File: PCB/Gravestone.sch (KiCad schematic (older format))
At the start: 30 parts, among them J1 USB_C_Receptacle_USB2.0, SW1 SW_PUSH, U1 ATmega32U2-AU, Y1 16MHz

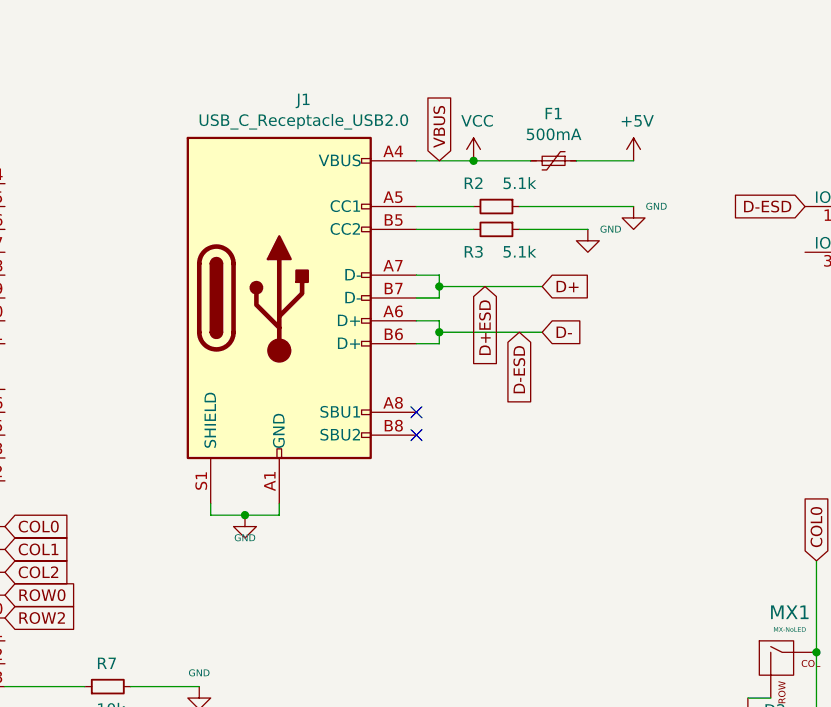
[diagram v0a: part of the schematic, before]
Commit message: 9/07 usb2
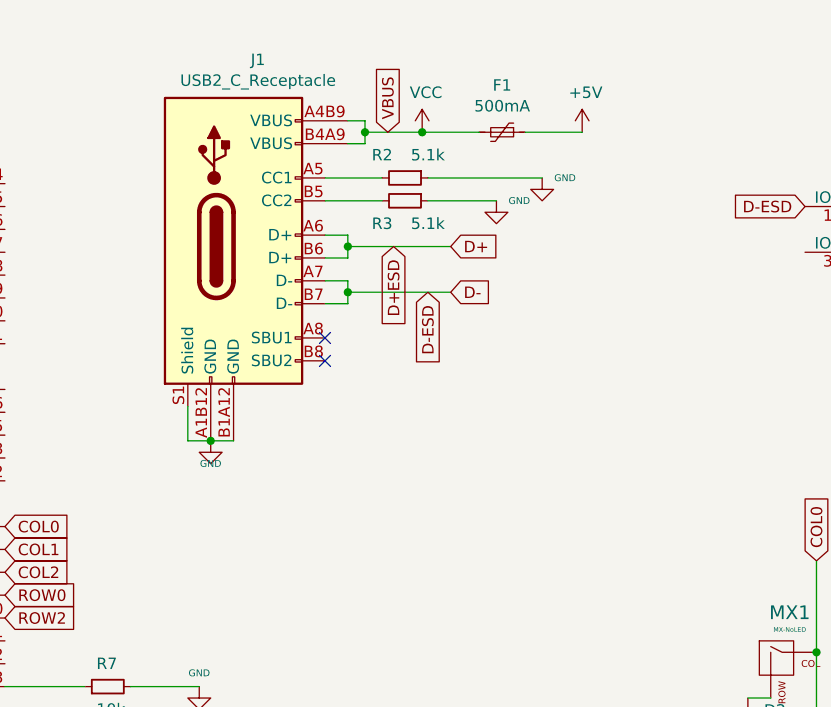
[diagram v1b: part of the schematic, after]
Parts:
- removed J1: USB_C_Receptacle_USB2.0, usb-type-c:Mid_Mount-USB_C_HandSoldering, symbol Connector:USB_C_Receptacle_USB2.0
- added J1: USB2_C_Receptacle, usb-type-c:Mid_Mount-USB_C_HandSoldering, symbol usb-type-c:USB2_C_Receptacle
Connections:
- net D+: now also J1.A6 (D+), J1.B6 (D+)
- net D-: now also J1.A7 (D-), J1.B7 (D-)
- net GND: now also J1.A1B12 (GND), J1.B1A12 (GND), J1.S1 (Shield)
- net VCC: now also J1.A4B9 (VBUS), J1.B4A9 (VBUS)
- net at R2.2: now also J1.A5 (CC1)
- net at R3.2: now also J1.B5 (CC2)
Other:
- moved on the sheet: F1, R2, R3
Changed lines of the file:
@@
 L Device:R_Small R2
 U 1 1 5F466C25
-P 6050 1650
-F 0 "R2" V 5950 1550 50  0000 C CNN
-F 1 "5.1k" V 5950 1750 50  0000 C CNN
-F 2 "Keebio-Parts:R_0603" H 6050 1650 50  0001 C CNN
-F 3 "~" H 6050 1650 50  0001 C CNN
-	1    6050 1650
+P 5650 1525
+F 0 "R2" V 5550 1425 50  0000 C CNN
+F 1 "5.1k" V 5550 1625 50  0000 C CNN
+F 2 "Keebio-Parts:R_0603" H 5650 1525 50  0001 C CNN
+F 3 "~" H 5650 1525 50  0001 C CNN
+	1    5650 1525
 	0    1    1    0
 $EndComp
@@
 	2400 1250 2400 1150
 $Comp
-L Connector:USB_C_Receptacle_USB2.0 J1
-U 1 1 5F45EACB
-P 5100 2050
-F 0 "J1" H 5207 2917 50  0000 C CNN
-F 1 "USB_C_Receptacle_USB2.0" H 5207 2826 50  0000 C CNN
-F 2 "usb-type-c:Mid_Mount-USB_C_HandSoldering" H 5250 2050 50  0001 C CNN
-F 3 "https://www.usb.org/sites/default/files/documents/usb_type-c.zip" H 5250 2050 50  0001 C CNN
-	1    5100 2050
-	1    0    0    -1
-$EndComp
-$Comp
 L power:GND #PWR0111
 U 1 1 5F461E03
-P 4950 3000
-F 0 "#PWR0111" H 4950 3050 20  0001 C CNN
-F 1 "GND" H 4950 2900 30  0000 C CNN
-F 2 "" H 4950 3000 60  0000 C CNN
-F 3 "" H 4950 3000 60  0000 C CNN
-	1    4950 3000
+P 4800 2675
+F 0 "#PWR0111" H 4800 2725 20  0001 C CNN
+F 1 "GND" H 4800 2575 30  0000 C CNN
+F 2 "" H 4800 2675 60  0000 C CNN
+F 3 "" H 4800 2675 60  0000 C CNN
+	1    4800 2675
 	1    0    0    -1
 $EndComp
@@
 L power:VCC #PWR0112
 U 1 1 5F46330E
-P 5950 1450
-F 0 "#PWR0112" H 5950 1300 50  0001 C CNN
-F 1 "VCC" H 5967 1623 50  0000 C CNN
-F 2 "" H 5950 1450 50  0001 C CNN
-F 3 "" H 5950 1450 50  0001 C CNN
-	1    5950 1450
+P 5725 1325
+F 0 "#PWR0112" H 5725 1175 50  0001 C CNN
+F 1 "VCC" H 5742 1498 50  0000 C CNN
+F 2 "" H 5725 1325 50  0001 C CNN
+F 3 "" H 5725 1325 50  0001 C CNN
+	1    5725 1325
 	1    0    0    -1
 $EndComp
@@
 L Device:Polyfuse_Small F1
 U 1 1 5F464504
-P 6300 1450
-F 0 "F1" V 6095 1450 50  0000 C CNN
-F 1 "500mA" V 6186 1450 50  0000 C CNN
-F 2 "Fuse:Fuse_0805_2012Metric" H 6350 1250 50  0001 L CNN
-F 3 "~" H 6300 1450 50  0001 C CNN
-	1    6300 1450
+P 6075 1325
+F 0 "F1" V 5870 1325 50  0000 C CNN
+F 1 "500mA" V 5961 1325 50  0000 C CNN
+F 2 "Fuse:Fuse_0805_2012Metric" H 6125 1125 50  0001 L CNN
+F 3 "~" H 6075 1325 50  0001 C CNN
+	1    6075 1325
 	0    1    1    0
 $EndComp
@@
 L power:+5V #PWR0113
 U 1 1 5F465DF5
-P 6650 1450
-F 0 "#PWR0113" H 6650 1300 50  0001 C CNN
-F 1 "+5V" H 6665 1623 50  0000 C CNN
-F 2 "" H 6650 1450 50  0001 C CNN
-F 3 "" H 6650 1450 50  0001 C CNN
-	1    6650 1450
-	1    0    0    -1
-$EndComp
-Wire Wire Line
-	5700 1450 5950 1450
-Wire Wire Line
-	6400 1450 6650 1450
-Connection ~ 5950 1450
-Wire Wire Line
-	5950 1450 6200 1450
+P 6425 1325
+F 0 "#PWR0113" H 6425 1175 50  0001 C CNN
+F 1 "+5V" H 6440 1498 50  0000 C CNN
+F 2 "" H 6425 1325 50  0001 C CNN
+F 3 "" H 6425 1325 50  0001 C CNN
+	1    6425 1325
+	1    0    0    -1
+$EndComp
+Wire Wire Line
+	5475 1325 5725 1325
+Wire Wire Line
+	6175 1325 6425 1325
+Connection ~ 5725 1325
+Wire Wire Line
+	5725 1325 5975 1325
 $Comp
 L Device:R_Small R3
 U 1 1 5F468C9D
-P 6050 1750
-F 0 "R3" V 6150 1650 50  0000 C CNN
-F 1 "5.1k" V 6150 1850 50  0000 C CNN
-F 2 "Keebio-Parts:R_0603" H 6050 1750 50  0001 C CNN
-F 3 "~" H 6050 1750 50  0001 C CNN
-	1    6050 1750
-	0    1    1    0
-$EndComp
-Wire Wire Line
-	5700 1650 5950 1650
-Wire Wire Line
-	5700 1750 5950 1750
+P 5650 1625
+F 0 "R3" V 5750 1525 50  0000 C CNN
+F 1 "5.1k" V 5750 1725 50  0000 C CNN
+F 2 "Keebio-Parts:R_0603" H 5650 1625 50  0001 C CNN
+F 3 "~" H 5650 1625 50  0001 C CNN
+	1    5650 1625
+	0    1    1    0
+$EndComp
+Wire Wire Line
+	5300 1525 5550 1525
+Wire Wire Line
+	5300 1625 5550 1625
 $Comp
 L Power_Protection:SRV05-4 D1
@@
 $EndComp
 Wire Wire Line
-	5700 1950 5800 1950
-Wire Wire Line
-	5800 2050 5700 2050
-Wire Wire Line
-	5700 2150 5800 2150
-Wire Wire Line
-	5800 2250 5700 2250
-Text GLabel 6250 2000 2    50   Input ~ 0
+	5300 1775 5400 1775
+Wire Wire Line
+	5400 1875 5300 1875
+Wire Wire Line
+	5300 1975 5400 1975
+Wire Wire Line
+	5400 2075 5300 2075
+Text GLabel 5850 1825 2    50   Input ~ 0
 D+
-Text GLabel 6250 2200 2    50   Input ~ 0
+Text GLabel 5850 2025 2    50   Input ~ 0
 D-
-NoConn ~ 5700 2550
-NoConn ~ 5700 2650
-Wire Wire Line
-	5100 2950 5100 3000
+NoConn ~ 5300 2225
+NoConn ~ 5300 2325
 $Comp
 L Gravestone-rescue:MX-NoLED-MX_Alps_Hybrid MX1
@@
 Wire Wire Line
 	3100 4150 3200 4150
-Wire Wire Line
-	4800 2950 4800 3000
 $Comp
 L power:GND #PWR0114
 U 1 1 5F56CBA5
-P 6650 1650
-F 0 "#PWR0114" H 6650 1700 20  0001 C CNN
-F 1 "GND" H 6750 1650 30  0000 C CNN
-F 2 "" H 6650 1650 60  0000 C CNN
-F 3 "" H 6650 1650 60  0000 C CNN
-	1    6650 1650
-	1    0    0    -1
-$EndComp
-Wire Wire Line
-	4800 3000 4950 3000
-Connection ~ 4950 3000
-Wire Wire Line
-	4950 3000 5100 3000
-Text GLabel 5800 1450 1    50   Input ~ 0
+P 6250 1525
+F 0 "#PWR0114" H 6250 1575 20  0001 C CNN
+F 1 "GND" H 6350 1525 30  0000 C CNN
+F 2 "" H 6250 1525 60  0000 C CNN
+F 3 "" H 6250 1525 60  0000 C CNN
+	1    6250 1525
+	1    0    0    -1
+$EndComp
+Text GLabel 5575 1325 1    50   Input ~ 0
 VBUS
 Wire Wire Line
-	5800 1950 5800 2000
-Wire Wire Line
-	5800 2150 5800 2200
+	5400 1775 5400 1825
+Wire Wire Line
+	5400 1975 5400 2025
 $Comp
 L power:GND #PWR0115
 U 1 1 5F48A564
-P 6450 1750
-F 0 "#PWR0115" H 6450 1800 20  0001 C CNN
-F 1 "GND" H 6550 1750 30  0000 C CNN
-F 2 "" H 6450 1750 60  0000 C CNN
-F 3 "" H 6450 1750 60  0000 C CNN
-	1    6450 1750
-	1    0    0    -1
-$EndComp
-Wire Wire Line
-	6150 1650 6650 1650
-Wire Wire Line
-	6150 1750 6450 1750
-Connection ~ 5800 2000
-Wire Wire Line
-	5800 2000 5800 2050
-Connection ~ 5800 2200
-Wire Wire Line
-	5800 2200 5800 2250
-Text GLabel 6150 2200 3    50   Input ~ 0
+P 6050 1625
+F 0 "#PWR0115" H 6050 1675 20  0001 C CNN
+F 1 "GND" H 6150 1625 30  0000 C CNN
+F 2 "" H 6050 1625 60  0000 C CNN
+F 3 "" H 6050 1625 60  0000 C CNN
+	1    6050 1625
+	1    0    0    -1
+$EndComp
+Wire Wire Line
+	5750 1525 6250 1525
+Wire Wire Line
+	5750 1625 6050 1625
+Connection ~ 5400 1825
+Wire Wire Line
+	5400 1825 5400 1875
+Connection ~ 5400 2025
+Wire Wire Line
+	5400 2025 5400 2075
+Text GLabel 5750 2025 3    50   Input ~ 0
 D-ESD
-Text GLabel 6000 2000 3    50   Input ~ 0
+Text GLabel 5600 1825 3    50   Input ~ 0
 D+ESD
 Wire Wire Line
-	5800 2000 6250 2000
-Wire Wire Line
-	5800 2200 6250 2200
+	5400 1825 5850 1825
+Wire Wire Line
+	5400 2025 5850 2025
 Text GLabel 7400 1650 0    50   Input ~ 0
 D-ESD
@@
 Wire Wire Line
 	4950 4275 5350 4275
+$Comp
+L usb-type-c:USB2_C_Receptacle J1
+U 1 1 5F5657E8
+P 4900 1825
+F 0 "J1" H 5007 2642 50  0000 C CNN
+F 1 "USB2_C_Receptacle" H 5007 2551 50  0000 C CNN
+F 2 "usb-type-c:Mid_Mount-USB_C_HandSoldering" H 5100 1875 50  0001 C CNN
+F 3 " ~" H 5100 1875 50  0001 C CNN
+	1    4900 1825
+	1    0    0    -1
+$EndComp
+Wire Wire Line
+	4900 2675 4800 2675
+Connection ~ 4800 2675
+Wire Wire Line
+	4800 2675 4700 2675
+Wire Wire Line
+	4700 2675 4700 2525
+Wire Wire Line
+	5400 1275 5475 1275
+Wire Wire Line
+	5475 1275 5475 1325
+Wire Wire Line
+	5475 1375 5400 1375
+Connection ~ 5475 1325
+Wire Wire Line
+	5475 1325 5475 1375
 $EndSCHEMATC

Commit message: 9/7 1021
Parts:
- C1, C2, C4, C5, C6, C7: symbol Device:C_Small -> Gravestone-rescue:C_Small-Device
- D1: symbol Power_Protection:SRV05-4 -> Gravestone-rescue:SRV05-4-Power_Protection
- D2, D3, D4, D5, D6, D7: symbol Device:D_Small -> Gravestone-rescue:D_Small-Device
- F1: symbol Device:Polyfuse_Small -> Gravestone-rescue:Polyfuse_Small-Device
- R1, R2, R3, R4, R5, R7: symbol Device:R_Small -> Gravestone-rescue:R_Small-Device
- SW1: symbol Switch:SW_Push -> Gravestone-rescue:SW_Push-Switch
- Y1: symbol Device:Crystal_GND24_Small -> Gravestone-rescue:Crystal_GND24_Small-Device
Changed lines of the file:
@@
 $EndDescr
 $Comp
-L Device:R_Small R2
+L Gravestone-rescue:R_Small-Device R2
 U 1 1 5F466C25
 P 5650 1525
@@
 $EndComp
 $Comp
-L Device:C_Small C7
+L Gravestone-rescue:C_Small-Device C7
 U 1 1 5F46A94B
 P 2150 2700
@@
 	2150 2800 2150 2900
 $Comp
-L Device:Crystal_GND24_Small Y1
+L Gravestone-rescue:Crystal_GND24_Small-Device Y1
 U 1 1 5F4740EB
 P 1900 1850
@@
 	1900 1950 2500 1950
 $Comp
-L Device:C_Small C1
+L Gravestone-rescue:C_Small-Device C1
 U 1 1 5F47A0E6
 P 1600 1650
@@
 $EndComp
 $Comp
-L Device:C_Small C2
+L Gravestone-rescue:C_Small-Device C2
 U 1 1 5F47B088
 P 1600 2050
@@
 Connection ~ 1500 2150
 $Comp
-L Switch:SW_Push SW1
+L Gravestone-rescue:SW_Push-Switch SW1
 U 1 1 5F480596
 P 2100 1550
@@
 $EndComp
 $Comp
-L Device:R_Small R1
+L Gravestone-rescue:R_Small-Device R1
 U 1 1 5F4821C1
 P 2400 1350
@@
 $EndComp
 $Comp
-L Device:Polyfuse_Small F1
+L Gravestone-rescue:Polyfuse_Small-Device F1
 U 1 1 5F464504
 P 6075 1325
@@
 	5725 1325 5975 1325
 $Comp
-L Device:R_Small R3
+L Gravestone-rescue:R_Small-Device R3
 U 1 1 5F468C9D
 P 5650 1625
@@
 	5300 1625 5550 1625
 $Comp
-L Power_Protection:SRV05-4 D1
+L Gravestone-rescue:SRV05-4-Power_Protection D1
 U 1 1 5F46CDD8
 P 7900 1750
@@
 $EndComp
 $Comp
-L Device:D_Small D2
+L Gravestone-rescue:D_Small-Device D2
 U 1 1 5F45B72E
 P 7150 3900
@@
 $EndComp
 $Comp
-L Device:D_Small D3
+L Gravestone-rescue:D_Small-Device D3
 U 1 1 5F45E94F
 P 7700 3900
@@
 $EndComp
 $Comp
-L Device:D_Small D4
+L Gravestone-rescue:D_Small-Device D4
 U 1 1 5F460C2A
 P 8250 3900
@@
 $EndComp
 $Comp
-L Device:D_Small D5
+L Gravestone-rescue:D_Small-Device D5
 U 1 1 5F465166
 P 7150 4600
@@
 $EndComp
 $Comp
-L Device:D_Small D6
+L Gravestone-rescue:D_Small-Device D6
 U 1 1 5F465173
 P 7700 4600
@@
 $EndComp
 $Comp
-L Device:D_Small D7
+L Gravestone-rescue:D_Small-Device D7
 U 1 1 5F465180
 P 8250 4600
@@
 $EndComp
 $Comp
-L Device:R_Small R7
+L Gravestone-rescue:R_Small-Device R7
 U 1 1 5F47354A
 P 4350 3750
@@
 Connection ~ 5350 4075
 $Comp
-L Device:C_Small C6
+L Gravestone-rescue:C_Small-Device C6
 U 1 1 5F46FC63
 P 5700 4175
@@
 $EndComp
 $Comp
-L Device:C_Small C5
+L Gravestone-rescue:C_Small-Device C5
 U 1 1 5F46E053
 P 5350 4175
@@
 $EndComp
 $Comp
-L Device:C_Small C4
+L Gravestone-rescue:C_Small-Device C4
 U 1 1 5F46CEE3
 P 4950 4175
@@
 $EndComp
 $Comp
-L Device:R_Small R4
+L Gravestone-rescue:R_Small-Device R4
 U 1 1 5F4686CC
 P 1750 2300
@@
 $EndComp
 $Comp
-L Device:R_Small R5
+L Gravestone-rescue:R_Small-Device R5
 U 1 1 5F46911B
 P 1750 2400
